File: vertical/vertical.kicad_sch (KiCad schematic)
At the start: 15 parts, among them J1 internal, J2 PROG, U1 LM1117-3.3, U2 ESP32-C3-WROOM-02, U5 MAX485E

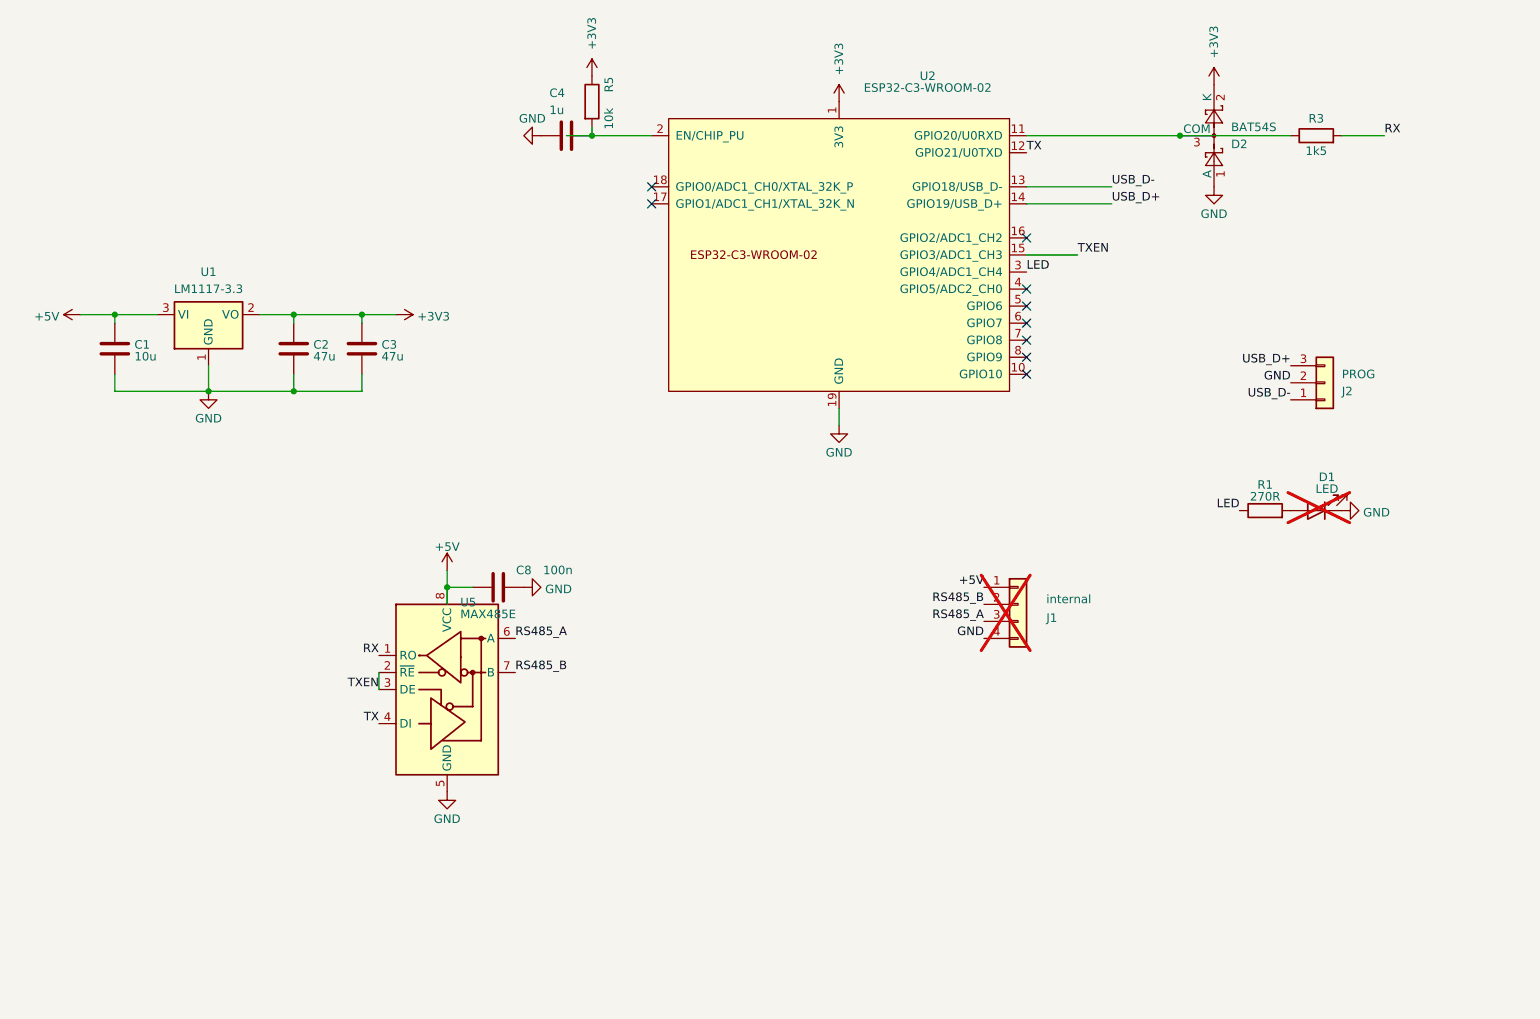
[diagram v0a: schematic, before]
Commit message: Update KiCad design files
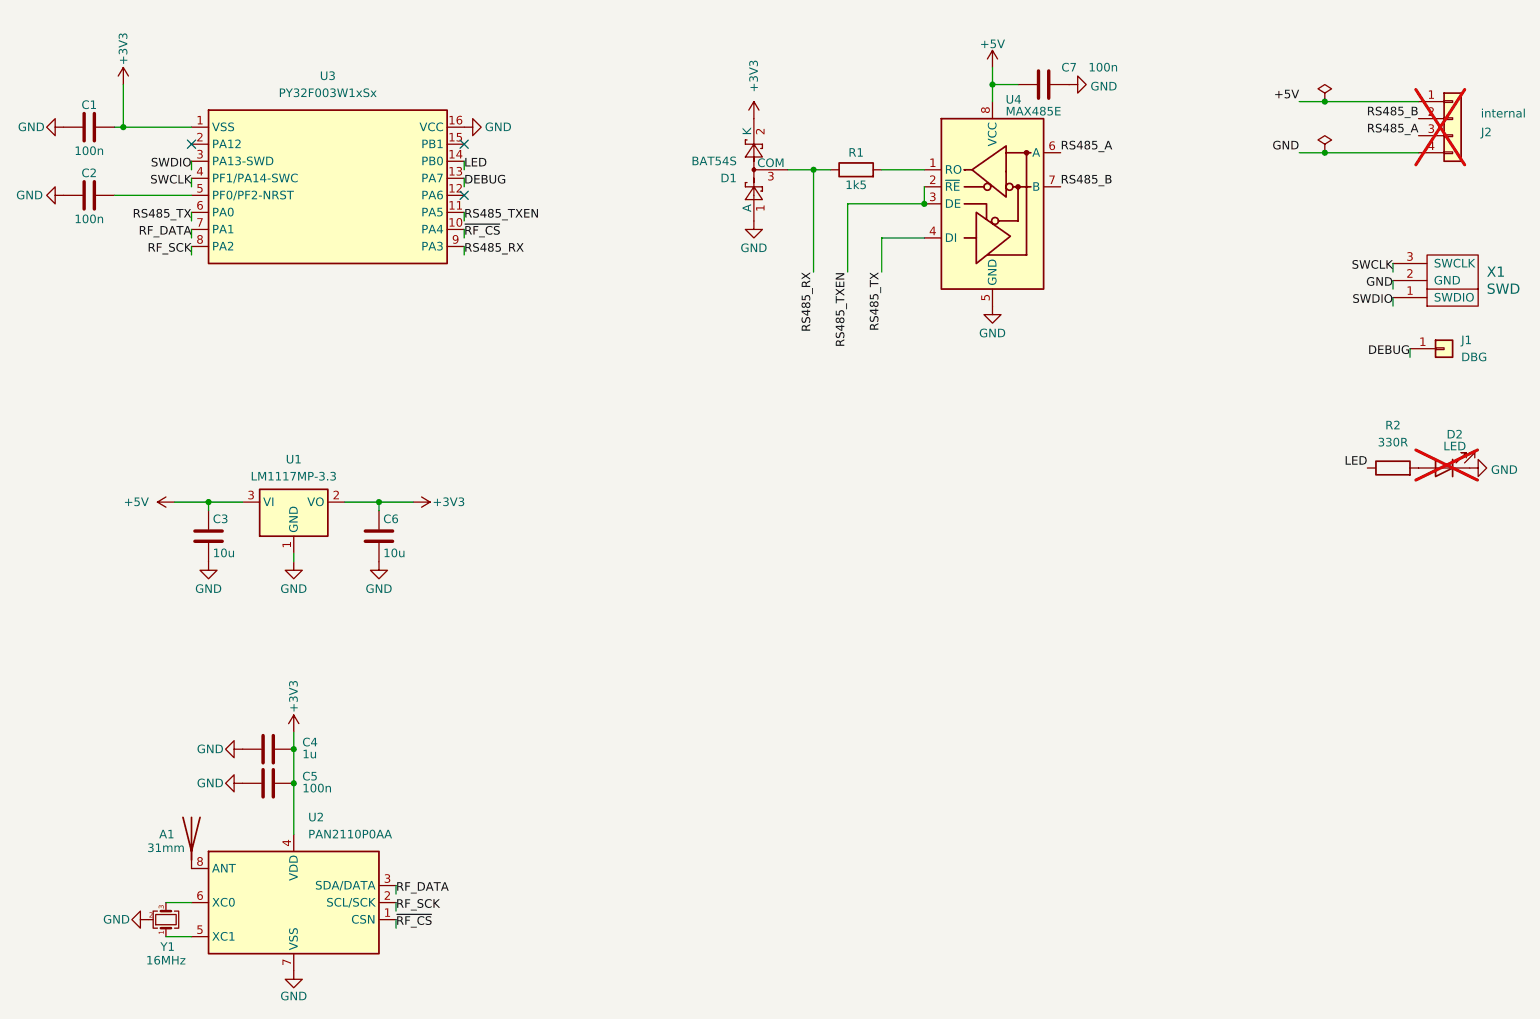
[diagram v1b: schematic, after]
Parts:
- removed J2: PROG, Connector_PinHeader_2.54mm:PinHeader_1x03_P2.54mm_Vertical, symbol Connector_Generic:Conn_01x03
- removed R5: 10k, Resistor_SMD:R_0805_2012Metric_Pad1.20x1.40mm_HandSolder, symbol Device:R
- removed U2: ESP32-C3-WROOM-02, Drake:ESP32-C3-WROOM-02-Handsolder, symbol Espressif:ESP32-C3-WROOM-02
- added A1: 31mm, Drake:Wire antena 2.4GHz, symbol Device:Antenna
- added C5: 100n, Capacitor_SMD:C_0805_2012Metric, symbol Device:C
- added C6: 10u, Capacitor_SMD:C_0805_2012Metric, symbol Device:C
- added J1: DBG, Connector_PinHeader_2.54mm:PinHeader_1x01_P2.54mm_Vertical, symbol Connector_Generic:Conn_01x01
- added U2: PAN2110P0AA, Package_SO:SOIC-8_3.9x4.9mm_P1.27mm, symbol Drake:PAN2110P0AA
- added U3: PY32F003W1xSx, Package_SO:SOIC-16_3.9x9.9mm_P1.27mm, symbol MCU_Puya_PY32F:PY32F003W1xSx
- added X1: SWD, Drake:SWD, symbol Drake:SWD
- added Y1: 16MHz, Crystal:Crystal_SMD_3225-4Pin_3.2x2.5mm, symbol Device:Crystal_GND24_Small
- C1: value 10u -> 100n; footprint Capacitor_SMD:C_0805_2012Metric_Pad1.18x1.45mm_HandSolder -> Capacitor_SMD:C_0805_2012Metric
- C2: value 47u -> 100n; footprint Capacitor_SMD:C_0805_2012Metric_Pad1.18x1.45mm_HandSolder -> Capacitor_SMD:C_0805_2012Metric
- C3: value 47u -> 10u; footprint Capacitor_SMD:C_0805_2012Metric_Pad1.18x1.45mm_HandSolder -> Capacitor_SMD:C_0805_2012Metric
- C4: footprint Capacitor_SMD:C_0805_2012Metric_Pad1.18x1.45mm_HandSolder -> Capacitor_SMD:C_0805_2012Metric
- C7: renamed from C8; footprint Capacitor_SMD:C_0805_2012Metric_Pad1.18x1.45mm_HandSolder -> Capacitor_SMD:C_0805_2012Metric
- R1: renamed from R3; footprint Resistor_SMD:R_0805_2012Metric_Pad1.20x1.40mm_HandSolder -> Resistor_SMD:R_0805_2012Metric
- R2: renamed from R1; value 270R -> 330R; footprint Resistor_SMD:R_0805_2012Metric_Pad1.20x1.40mm_HandSolder -> Resistor_SMD:R_0805_2012Metric
- U1: value LM1117-3.3 -> LM1117MP-3.3
- renumbered D2 to D1, D1 to D2, J1 to J2, U5 to U4
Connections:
- net +3V3: now also C1.1, C4.1, C5.1, C6.1, U2.4 (VDD), U3.1 (VSS); no longer C2.1, C3.1
- net +5V: now also C3.1; no longer C1.1
- net GND: now also C5.2, C6.2, U2.7 (VSS), U3.16 (VCC), X1.2 (GND), Y1.2 (G), Y1.4 (G)
- net LED: now also U3.14 (PB0)
- net RS485_RX: now reaches D1.3 (COM), R1.1
- net RS485_RX: now also U3.9 (PA3)
- net RX: no longer names the net of R1.2, U4.1 (RO)
- net TX renamed RS485_TX
- net RS485_TX: now also U3.6 (PA0)
- net TXEN renamed RS485_TXEN
- net RS485_TXEN: now also U3.11 (PA5)
- new net: U2.5 (XC1), Y1.1
- new net: U2.6 (XC0), Y1.3
- new net: A1.1 (A), U2.8 (ANT)
- new net: C2.1, U3.5 (PF0/PF2-NRST)
- new net DEBUG: J1.1 (Pin_1), U3.13 (PA7)
- new net RF_DATA: U2.3 (SDA/DATA), U3.7 (PA1)
- new net RF_SCK: U2.2 (SCL/SCK), U3.8 (PA2)
- new net SWCLK: U3.4 (PF1/PA14-SWC), X1.3 (SWCLK)
- new net SWDIO: U3.3 (PA13-SWD), X1.1 (SWDIO)
- new net ~{RF_CS}: U2.1 (CSN), U3.10 (PA4)
- no-connect marks 9 -> 3
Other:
- moved on the sheet: C7, D1, D2, J2, R1, R2, U4
